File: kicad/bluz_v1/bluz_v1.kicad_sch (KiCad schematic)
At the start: 61 parts, among them J1 USB_B_Micro, J11 Conn, J12 BTAnt, J2 Conn, J3 Conn, J4 Conn, J5 Conn, J6 Conn, J7 Conn, J8 Conn, M1 VibroMotor, Q1 RUM002N05, Q2 RUM002N05, SW1 SW_DPDT_x2, U1 MCP73831, U2 MCP1700, U3 TLV3201AIDCK, U4 AP3015KTR, Y1 NX2016SA-32MHz

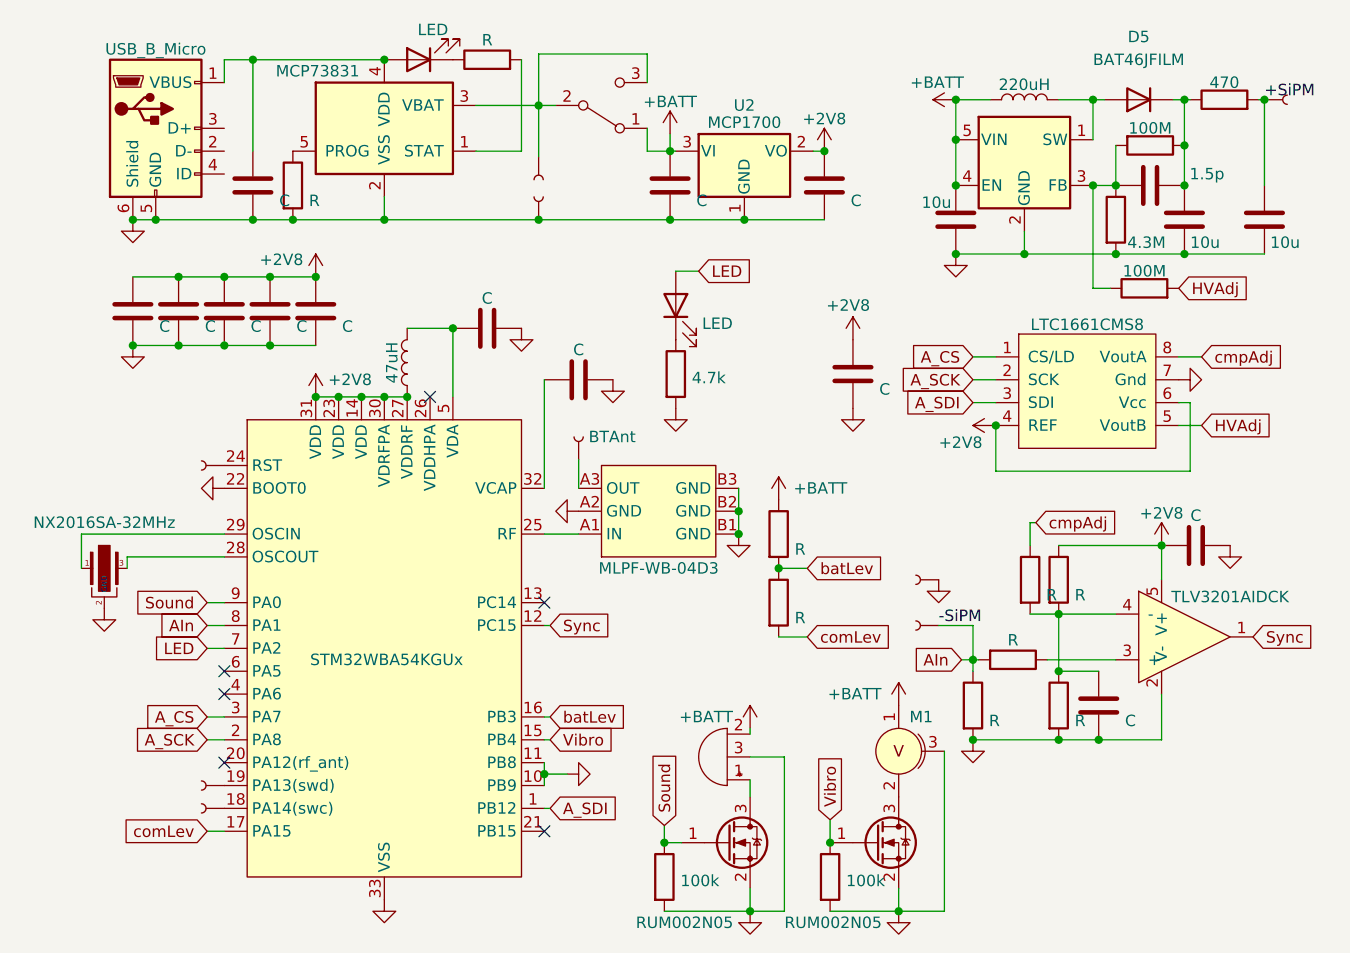
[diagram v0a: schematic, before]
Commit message: изменено:      Documents/BluZ.png 	удалено:       kicad/bluz_v1/bluz_v1-backups/bluz_v1-2024-05-03_150608.zip 	удалено:       kicad/bluz_v1/bluz_v1-backups/bluz_v1-2024-05-03_151512.zip 	удалено:       kicad/bluz_v1/bluz_v1-backups/bluz_v1-2024-05-03_172047.zip 	изменено:      kicad/bluz_v1/bluz_v1.kicad_pcb 	изменено:      kicad/bluz_v1/bluz_v1.kicad_sch 	изменено:      kicad/bluz_v1/fp-info-cache
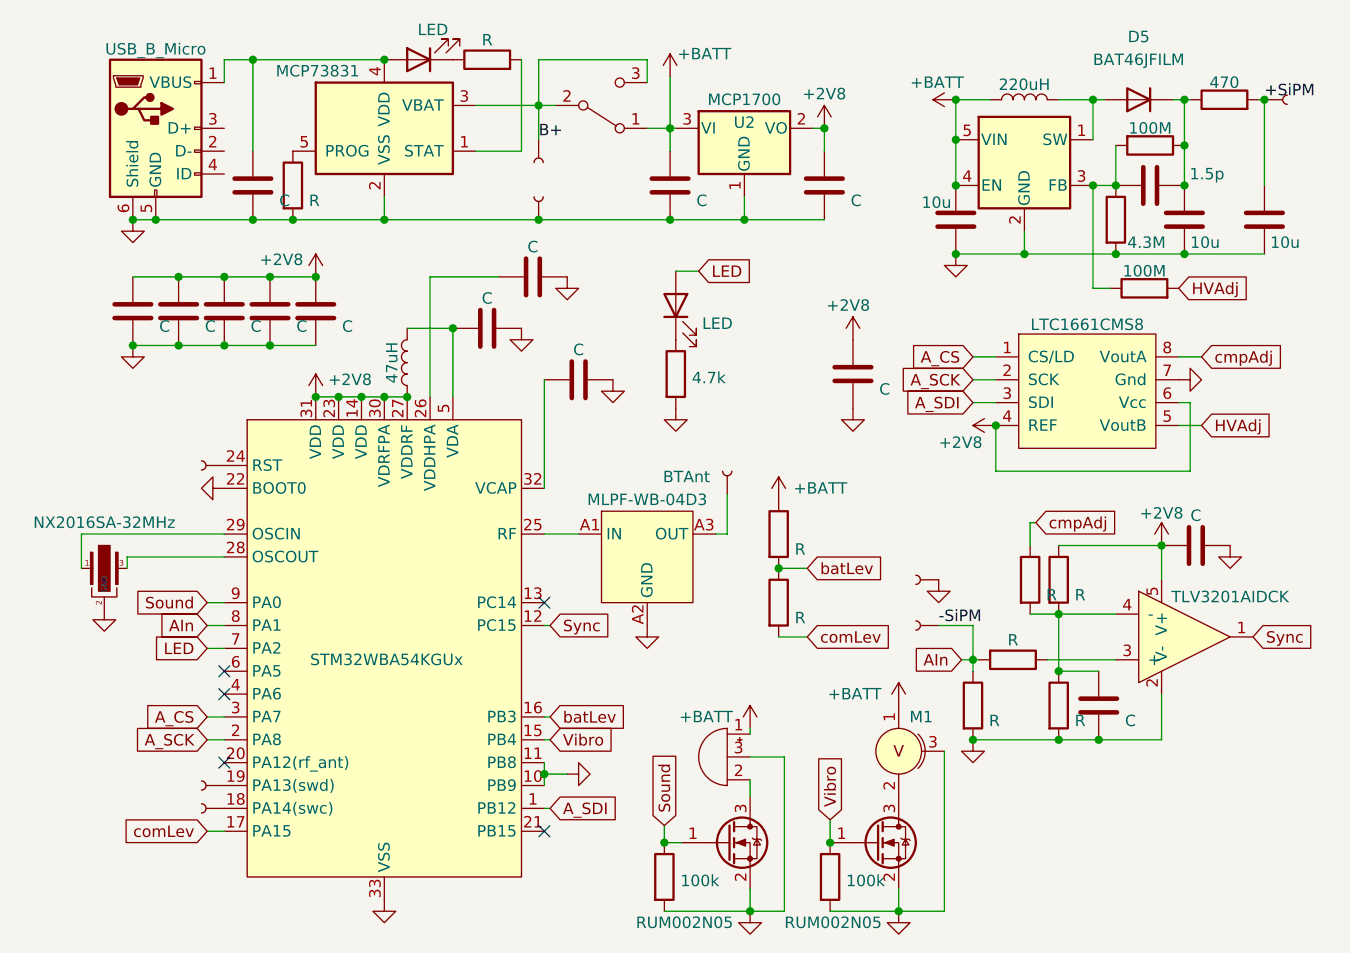
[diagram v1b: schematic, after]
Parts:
- added C17: C, Capacitor_SMD:C_0402_1005Metric, symbol Device:C
- R16: footprint Resistor_SMD:R_0603_1608Metric -> Resistor_SMD:R_0402_1005Metric
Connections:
- net +BATT: now also BZ1.1 (-); no longer BZ1.2 (+)
- net GND: now also C17.2
- net at Q1.3 (D): now also BZ1.2 (+); no longer BZ1.1 (-)
- net at D1.26 (VDDHPA): now also C17.1
- net B+: now reaches J6.1, SW1.2 (B), SW1.3 (C), U1.3 (VBAT)
- no-connect marks 6 -> 5
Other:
- moved on the sheet: U2
